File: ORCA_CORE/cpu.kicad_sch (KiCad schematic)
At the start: 48 parts, among them J10 Raspberry_Pi_2_3, J11 I2C, J12 I2C, J13 6Vout, J15 Conn_01x05_Pin, J16 Conn_01x05_Pin, J20 5Vout, P1 USB_C_Receptacle_USB2.0, Q6 BSS138, Q7 BSS138, Q8 BSS138, U13 FT230XS, U14 BNO055, U15 NJM78055DL1

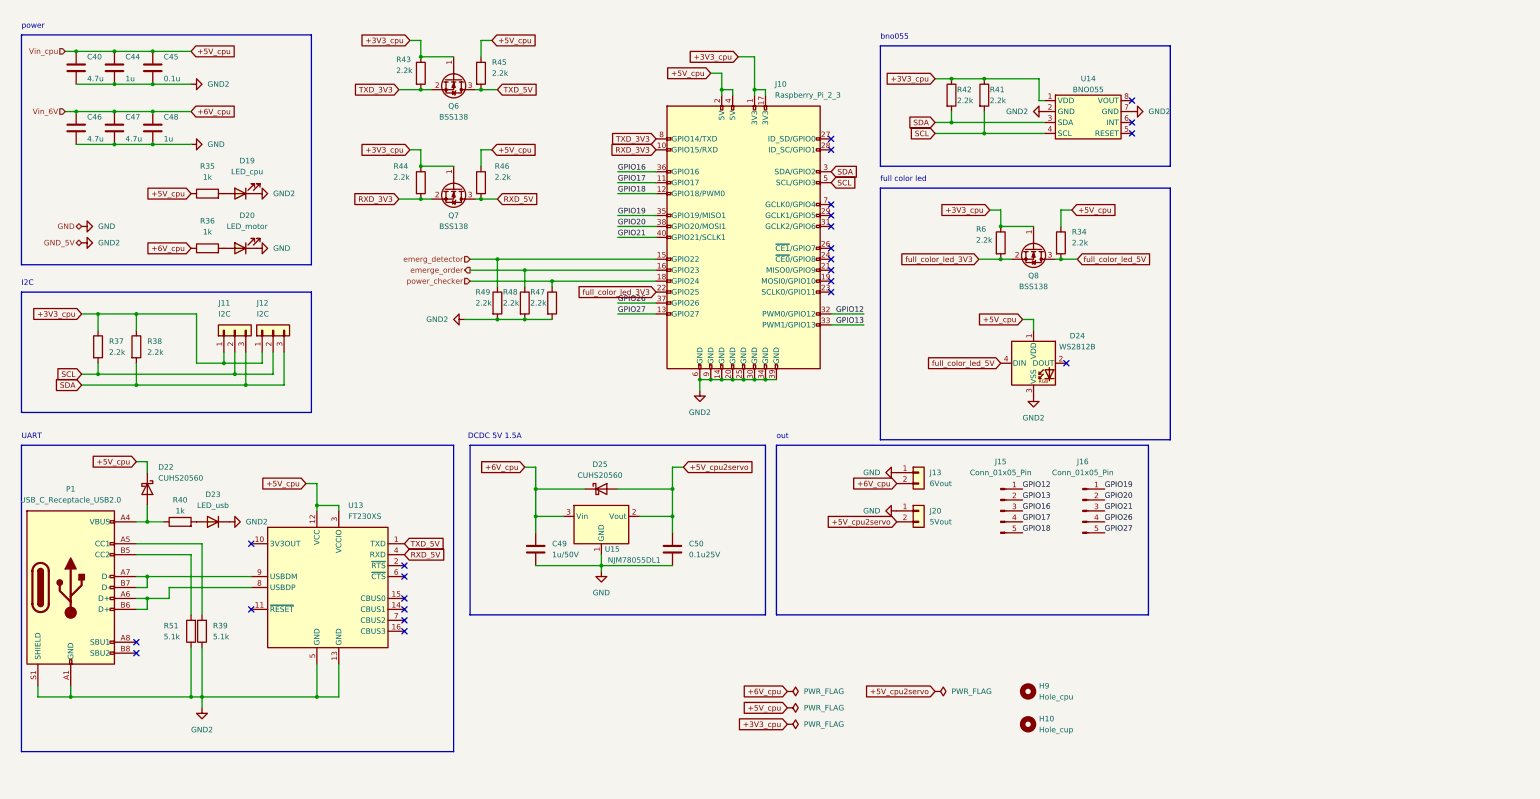
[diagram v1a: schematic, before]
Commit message: start making ORCA_CORE
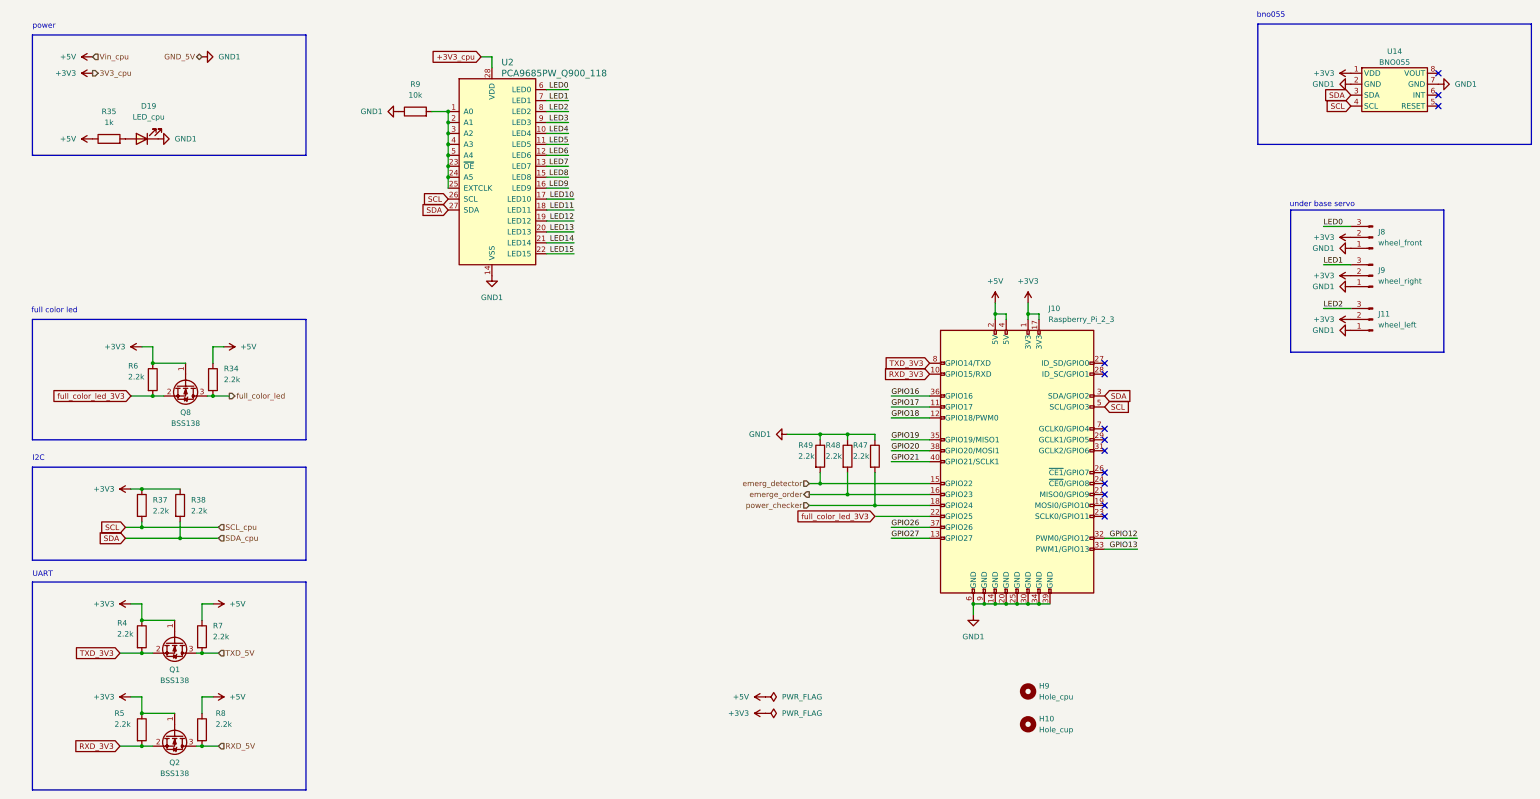
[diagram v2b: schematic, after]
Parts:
- removed C40, C46, C47: 4.7u, Capacitor_SMD:C_0603_1608Metric_Pad1.08x0.95mm_HandSolder, symbol Device:C
- removed C44, C48: 1u, Capacitor_SMD:C_0805_2012Metric_Pad1.18x1.45mm_HandSolder, symbol Device:C
- removed C45: 0.1u, Capacitor_SMD:C_0603_1608Metric_Pad1.08x0.95mm_HandSolder, symbol Device:C
- removed C49: 1u/50V, Capacitor_SMD:C_0805_2012Metric_Pad1.18x1.45mm_HandSolder, symbol Device:C
- removed C50: 0.1u25V, Capacitor_SMD:C_0603_1608Metric_Pad1.08x0.95mm_HandSolder, symbol Device:C
- removed D20: LED_motor, LED_SMD:LED_0603_1608Metric_Pad1.05x0.95mm_HandSolder, symbol Device:LED_Filled
- removed D22, D25: CUHS20560, Diode:Diode_US2H, symbol Device:D_Schottky
- removed D23: LED_usb, LED_SMD:LED_0603_1608Metric_Pad1.05x0.95mm_HandSolder, symbol Device:D_Filled
- removed D24: WS2812B, LED_SMD:LED_WS2812B_PLCC4_5.0x5.0mm_P3.2mm, symbol LED:WS2812B
- removed J11, J12: I2C, Connector_JST:JST_XH_B3B-XH-A_1x03_P2.50mm_Vertical, symbol Connector_Generic:Conn_01x03
- removed J13: 6Vout, Conn:power_pad, symbol Connector_Generic:Conn_01x02
- removed J15, J16: Conn_01x05_Pin, Connector_PinHeader_2.54mm:PinHeader_1x05_P2.54mm_Vertical, symbol Connector:Conn_01x05_Pin
- removed J20: 5Vout, Conn:power_pad, symbol Connector_Generic:Conn_01x02
- removed P1: USB_C_Receptacle_USB2.0, Conn:USB_C_Receptacle_XKB_U262-16XN-4BVC11, symbol Connector:USB_C_Receptacle_USB2.0
- removed Q6, Q7: BSS138, Package_TO_SOT_SMD:SOT-23, symbol Transistor_FET:BSS138
- removed R36, R40: 1k, Resistor_SMD:R_0603_1608Metric_Pad0.98x0.95mm_HandSolder, symbol Device:R
- removed R39, R51: 5.1k, Resistor_SMD:R_0603_1608Metric_Pad0.98x0.95mm_HandSolder, symbol Device:R
- removed R41, R42, R43, R44, R45, R46: 2.2k, Resistor_SMD:R_0603_1608Metric_Pad0.98x0.95mm_HandSolder, symbol Device:R
- removed U13: FT230XS, Package_SO:SSOP-16_3.9x4.9mm_P0.635mm, symbol Interface_USB:FT230XS
- removed U15: NJM78055DL1, Package_TO_SOT_SMD:TO-252-2, symbol mylib:NJM7805SDL1
- added J11: wheel_left, symbol Connector:Conn_01x03_Pin
- added J8: wheel_front, symbol Connector:Conn_01x03_Pin
- added J9: wheel_right, symbol Connector:Conn_01x03_Pin
- added Q1, Q2: BSS138, Package_TO_SOT_SMD:SOT-23, symbol Transistor_FET:BSS138
- added R4, R5, R7, R8: 2.2k, Resistor_SMD:R_0603_1608Metric_Pad0.98x0.95mm_HandSolder, symbol Device:R
- added R9: 10k, symbol Device:R
- added U2: PCA9685PW_Q900_118, digikey-footprints:TSSOP-28_W4.40mm, symbol dk_PMIC-LED-Drivers:PCA9685PW_Q900_118
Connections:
- net +3V3_cpu: now also U2.28 (VDD); no longer J10.1 (3V3), J10.17 (3V3), Q8.1 (G), R37.1, R38.1, R6.1, U14.1 (VDD)
- net RXD_3V3: now also Q2.2 (S), R5.2
- net RXD_5V: now also Q2.3 (D), R8.2
- net SCL: now also U2.26 (SCL)
- net SDA: now also U2.27 (SDA)
- net TXD_3V3: now also Q1.2 (S), R4.2
- net TXD_5V: now also Q1.3 (D), R7.2
- net emerg_detector: now also R49.2; no longer R49.1
- net emerge_order: now also R48.2; no longer R48.1
- net power_checker: now also R47.2; no longer R47.1
- net +5V_cpu renamed +5V
- net +5V: now also R7.1, R8.1
- net GND2 renamed GND1
- net GND1: now also R47.1, R48.1, R49.1, J11.1 (Pin_1), J8.1 (Pin_1), J9.1 (Pin_1), R9.1, U2.14 (VSS); no longer R47.2, R48.2, R49.2
- net full_color_led_5V renamed full_color_led
- new net: R9.2, U2.1 (A0), U2.2 (A1), U2.23 (~{OE}), U2.24 (A5), U2.25 (EXTCLK), U2.3 (A2), U2.4 (A3), U2.5 (A4)
- new net +3V3: J10.1 (3V3), J10.17 (3V3), J11.2 (Pin_2), J8.2 (Pin_2), J9.2 (Pin_2), Q1.1 (G), Q2.1 (G), Q8.1 (G), R37.1, R38.1, R4.1, R5.1, R6.1, U14.1 (VDD)
- new net LED0: J8.3 (Pin_3), U2.6 (LED0)
- new net LED1: J9.3 (Pin_3), U2.7 (LED1)
- new net LED10: U2.17 (LED10)
- new net LED11: U2.18 (LED11)
- new net LED12: U2.19 (LED12)
- new net LED13: U2.20 (LED13)
- new net LED14: U2.21 (LED14)
- new net LED15: U2.22 (LED15)
- new net LED2: J11.3 (Pin_3), U2.8 (LED2)
- new net LED3: U2.9 (LED3)
- new net LED4: U2.10 (LED4)
- new net LED5: U2.11 (LED5)
- new net LED6: U2.12 (LED6)
- new net LED7: U2.13 (LED7)
- new net LED8: U2.15 (LED8)
- new net LED9: U2.16 (LED9)
- no-connect marks 24 -> 13
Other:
- note added: "under base servo"
- note removed: "DCDC 5V 1.5A"
- note removed: "out"
- moved on the sheet: D19, J10, Q8, R34, R35, R37, R38, R47, R48, R49, R6, U14
